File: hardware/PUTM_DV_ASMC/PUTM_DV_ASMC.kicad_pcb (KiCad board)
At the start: 4 copper layers, 90.4 x 95 mm, 184 parts, among them IC1 BTS722204ESAXUMA1, IC2 BTS722204ESAXUMA1, J1 FTSH-107-01-L-D-K, J2 IPBS-110-01-XX-D-GP, J4 74650073R, J5 74650073R, K2 FINDER-32.21-x000, Q1 30V/5A, Q2 BUK6D210, Q3 BUK6D210, Q4 BUK6D210, Q5 BUK6D210, T1 TP_VCC, T2 TP_+5V, T3 TP_+3V3, T4 TP_GND, T5 TP_GND, T6 TP_VCC, T7 TP_GND, T8 TP_+5V, T9 TP_GND, U1 LM4040C33FTA, U14 FODM217B, U15 FODM217B, U2 STM32G484RETx, U3 LM1117-3.3, U4 TPS54202HDDCR, U5 ADM3057ExRW, U6 ADM3057ExRW, Y1 ATX-11-F-32.000MHZ-F05-T

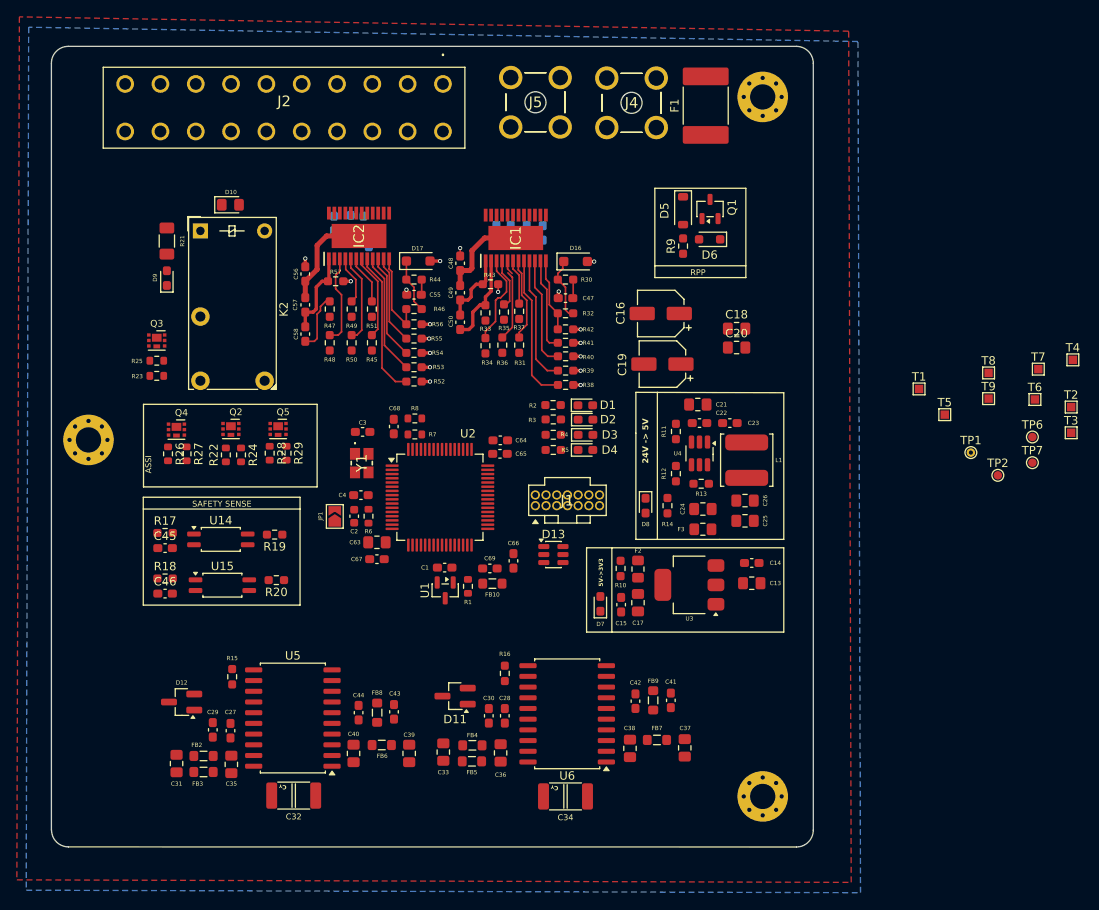
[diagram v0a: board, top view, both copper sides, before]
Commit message: work on supply and zones
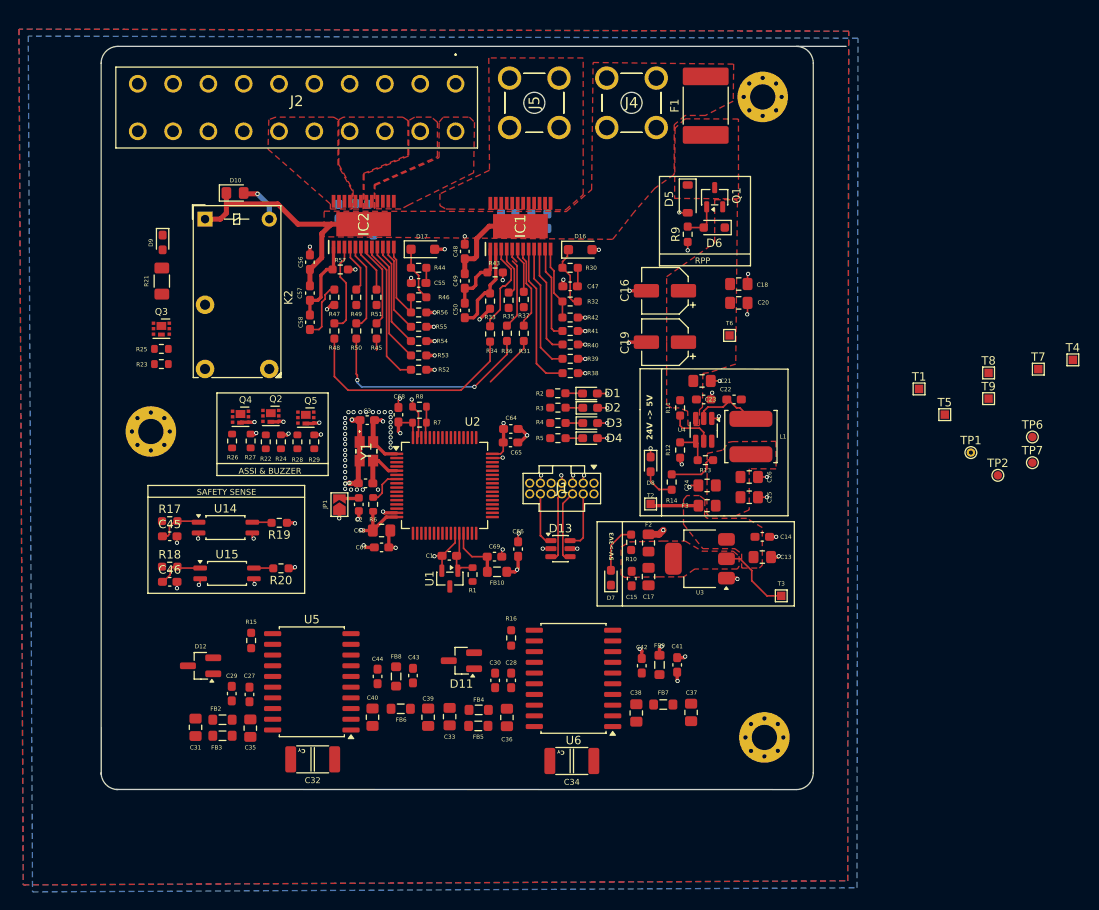
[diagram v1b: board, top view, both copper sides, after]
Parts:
- moved T2 51.2 mm to (192.0, 75.0)
- moved T3 39.5 mm to (207.5, 85.9)
- moved T6 37.0 mm to (201.4, 55.0)
- moved Q4 7.75 mm to (143.3, 64.7)
- moved R26 7.75 mm to (142.3, 67.5)
- moved R27 7.75 mm to (144.5, 67.5)
- moved REF** 7.47 mm to (132.7, 66.4)
- moved REF** 7.00 mm to (205.5, 102.7)
- moved J5 5.74 mm to (181.1, 30.3), turned to 90 degrees
- moved C18 5.31 mm to (202.5, 48.9)
- moved C20 5.31 mm to (202.5, 51.1)
- moved Q2 4.98 mm to (146.9, 64.5)
- moved R22 4.98 mm to (146.3, 67.6)
- moved R24 4.98 mm to (148.1, 67.6)
- moved D8 4.94 mm to (192.0, 70.3)
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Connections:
- C3 pad 1: +3.3V -> +3V3
- C41 pad 1: +3.3V -> +3V3
- C43 pad 1: +3.3V -> +3V3
- C47 pad 1: /DV_power_supply/Odrive_power_supply/FUSE_IS0 -> /DV_power_supply/FUSE_IS0
- C51 pad 1: /DV_power_supply/Odrive_power_supply/ODRIVE_1 -> /Connectors/ODRIVE4
- C52 pad 1: /DV_power_supply/Odrive_power_supply/ODRIVE_2 -> /Connectors/ODRIVE4
- C53 pad 1: /DV_power_supply/Odrive_power_supply/ODRIVE_3 -> /Connectors/ODRIVE4
- C54 pad 1: /DV_power_supply/Odrive_power_supply/ODRIVE_4 -> /Connectors/ODRIVE4
- C55 pad 1: /DV_power_supply/Dv_power_supply_component/FUSE_IS1 -> /DV_power_supply/FUSE_IS1
- C63 pad 1: +3.3V -> +3V3
- C64 pad 1: +3.3V -> +3V3
- C65 pad 1: +3.3V -> +3V3
- C66 pad 1: +3.3V -> +3V3
- C67 pad 1: +3.3V -> +3V3
- C68 pad 1: +3.3V -> +3V3
- D1 pad 2: +3.3V -> +3V3
- D2 pad 2: +3.3V -> +3V3
- D3 pad 2: +3.3V -> +3V3
- D4 pad 2: +3.3V -> +3V3
- D9 pad 1: Net-(D10-A) -> GND
- FB10 pad 1: +3.3V -> +3V3
- FB8 pad 2: +3.3V -> +3V3
- FB9 pad 2: +3.3V -> +3V3
- IC1 pad 13: /DV_power_supply/Odrive_power_supply/ODRIVE_4 -> /Connectors/ODRIVE4
- IC1 pad 14: /DV_power_supply/Odrive_power_supply/ODRIVE_4 -> /Connectors/ODRIVE4
- IC1 pad 15: /DV_power_supply/Odrive_power_supply/ODRIVE_4 -> /Connectors/ODRIVE4
- IC1 pad 16: /DV_power_supply/Odrive_power_supply/ODRIVE_4 -> /Connectors/ODRIVE4
- IC1 pad 17: /DV_power_supply/Odrive_power_supply/ODRIVE_3 -> /Connectors/ODRIVE4
- IC1 pad 18: /DV_power_supply/Odrive_power_supply/ODRIVE_3 -> /Connectors/ODRIVE4
- IC1 pad 19: /DV_power_supply/Odrive_power_supply/ODRIVE_2 -> /Connectors/ODRIVE4
- IC1 pad 20: /DV_power_supply/Odrive_power_supply/ODRIVE_2 -> /Connectors/ODRIVE4
- IC1 pad 21: /DV_power_supply/Odrive_power_supply/ODRIVE_1 -> /Connectors/ODRIVE4
- IC1 pad 22: /DV_power_supply/Odrive_power_supply/ODRIVE_1 -> /Connectors/ODRIVE4
- IC1 pad 23: /DV_power_supply/Odrive_power_supply/ODRIVE_1 -> /Connectors/ODRIVE4
- IC1 pad 24: /DV_power_supply/Odrive_power_supply/ODRIVE_1 -> /Connectors/ODRIVE4
- J5 pad 1: /Connectors/ODRIVE_4 -> /Connectors/ODRIVE4
- J5 pad 2: /Connectors/ODRIVE_1 -> /Connectors/ODRIVE4
- J5 pad 3: /Connectors/ODRIVE_2 -> /Connectors/ODRIVE4
- J5 pad 4: /Connectors/ODRIVE_3 -> /Connectors/ODRIVE4
- R19 pad 1: +3.3V -> +3V3
- R20 pad 1: +3.3V -> +3V3
- R21 pad 1: +BATT -> /Connectors/RES_SAFETY_OUTPUT
- R30 pad 1: /DV_power_supply/Odrive_power_supply/FUSE_IS0 -> /DV_power_supply/FUSE_IS0
- R31 pad 1: /DV_power_supply/LHI.0 -> /DV_power_supply/LHI0
- R34 pad 1: /DV_power_supply/SPI.MISO -> /DV_power_supply/SPI1.MISO
- R35 pad 1: /DV_power_supply/SPI.MOSI -> /DV_power_supply/SPI1.MOSI
- R36 pad 1: /DV_power_supply/SPI.SCK -> /DV_power_supply/SPI1.SCK
- R37 pad 1: /DV_power_supply/SPI.NSS -> /DV_power_supply/SPI1.NSS
- R44 pad 1: /DV_power_supply/Dv_power_supply_component/FUSE_IS1 -> /DV_power_supply/FUSE_IS1
- R45 pad 1: /DV_power_supply/LHI.1 -> /DV_power_supply/LHI1
- R48 pad 1: /DV_power_supply/SPI.MISO -> /DV_power_supply/SPI1.MISO
- R49 pad 1: /DV_power_supply/SPI.MOSI -> /DV_power_supply/SPI1.MOSI
- R50 pad 1: /DV_power_supply/SPI.SCK -> /DV_power_supply/SPI1.SCK
- R51 pad 1: /DV_power_supply/SPI.NSS -> /DV_power_supply/SPI1.NSS
- R6 pad 1: +3.3V -> +3V3
- R7 pad 1: +3.3V -> +3V3
- U2 pad 1: +3.3V -> +3V3
- U2 pad 12: /Microcontroller/LHI.0 -> /DV_power_supply/LHI0
- U2 pad 13: /Microcontroller/LHI.1 -> /DV_power_supply/LHI1
- U2 pad 16: +3.3V -> +3V3
- U2 pad 19: /Microcontroller/SPI1_SCK -> /DV_power_supply/SPI1.SCK
- U2 pad 20: /Microcontroller/SPI1_MISO -> /DV_power_supply/SPI1.MISO
- U2 pad 21: /Microcontroller/SPI1_MOSI -> /DV_power_supply/SPI1.MOSI
- U2 pad 32: +3.3V -> +3V3
- U2 pad 40: /Microcontroller/FUSE_ISO.0 -> /DV_power_supply/FUSE_IS0
- U2 pad 41: /Microcontroller/FUSE_ISO.1 -> /DV_power_supply/FUSE_IS1
- U2 pad 42: /Microcontroller/SPI1_NSS -> /DV_power_supply/SPI1.NSS
- U2 pad 48: +3.3V -> +3V3
- U2 pad 64: +3.3V -> +3V3
- Y1 pad 4: +3.3V -> +3V3
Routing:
- net GND: track 16.6 -> 89.5 mm, vias 18 -> 100
- net +3V3: track 0.00 -> 42.1 mm, vias 0 -> 17
- net /DV_power_supply/SPI1.MISO: track 0.00 -> 27.4 mm
- net /DV_power_supply/SPI1.SCK: track 0.00 -> 26.4 mm, vias 0 -> 2
- net +BATT: track 23.4 -> 42.6 mm
- net /Power_supply/VO_+3.3V: track 0.00 -> 9.03 mm
- net /Connectors/SWCLK: track 0.00 -> 8.67 mm
- net /Connectors/SWO: track 0.00 -> 8.38 mm
- net /Power_supply/SW_+5V: track 0.00 -> 8.25 mm
- net /Connectors/SWDIO: track 0.00 -> 6.91 mm
- net +3.3VA: track 0.00 -> 6.81 mm
- net /Microcontroller/NRST: track 0.00 -> 6.62 mm
- net /Microcontroller/VREF: track 0.00 -> 6.53 mm
- net /DV_power_supply/LHI0: track 0.00 -> 6.47 mm
- net /Connectors/NRST: track 0.00 -> 6.47 mm
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- added copper zone on F.Cu, net +24V
- added copper zone on In1.Cu, net +24V
- added copper zone on In2.Cu, net +24V
- added copper zone on B.Cu, net +3V3
- added copper zone on In1.Cu, net +5V
- added copper zone on In2.Cu, net +5V
- added copper zone on F.Cu, net +BATT
- added copper zone on In1.Cu, net +BATT
- added copper zone on In2.Cu, net +BATT
- added copper zone on F.Cu, net /Connectors/ODRIVE4
- added copper zone on In1.Cu, net /Connectors/ODRIVE4
- added copper zone on In2.Cu, net /Connectors/ODRIVE4
- added copper zone on F.Cu, net /Connectors/OUT_ASSI
- added copper zone on In1.Cu, net /Connectors/OUT_ASSI
- added copper zone on In2.Cu, net /Connectors/OUT_ASSI
- added copper zone on F.Cu, net /Connectors/OUT_EBS
- added copper zone on In1.Cu, net /Connectors/OUT_EBS
- added copper zone on In2.Cu, net /Connectors/OUT_EBS
- added copper zone on F.Cu, net /Connectors/OUT_LIDAR
- added copper zone on In1.Cu, net /Connectors/OUT_LIDAR
- added copper zone on In2.Cu, net /Connectors/OUT_LIDAR
- added copper zone on F.Cu, net /Connectors/OUT_RES
- added copper zone on In1.Cu, net /Connectors/OUT_RES
- added copper zone on In2.Cu, net /Connectors/OUT_RES
- added copper zone on F.Cu, net /Power_supply/+5V_OUT
- added copper zone on In1.Cu, net /Power_supply/+5V_OUT
- added copper zone on In2.Cu, net /Power_supply/+5V_OUT
- added copper zone on F.Cu, net /Power_supply/RPP_D
- added copper zone on In1.Cu, net /Power_supply/RPP_D
- added copper zone on In2.Cu, net /Power_supply/RPP_D
- added copper zone on F.Cu, net /Power_supply/VO_+3.3V
- added copper zone on In1.Cu, net /Power_supply/VO_+3.3V
- added copper zone on In2.Cu, net /Power_supply/VO_+3.3V
- added copper zone on B.Cu, net GND
- added copper zone on F.Cu, net GND
- removed copper zone on B.Cu, net +3.3V
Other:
- board size 90.4 x 95 mm -> 88.4 x 88.2 mm
- board text added: "ASSI & BUZZER"
- board text removed: "ASSI"
